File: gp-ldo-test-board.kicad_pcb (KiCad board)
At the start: 2 copper layers, 38.1 x 25.4 mm, 58 parts, among them J1 Conn_01x03, J2 Conn_01x02, J3 Conn_01x06, J4 Conn_01x02, J5 Conn_01x06, J6 Conn_01x02, J7 Conn_01x02, J8 Conn_01x02, J9 Conn_01x02, Q1 Q_PMOS_GSD, U1 SLG46582, U2 SLG46582

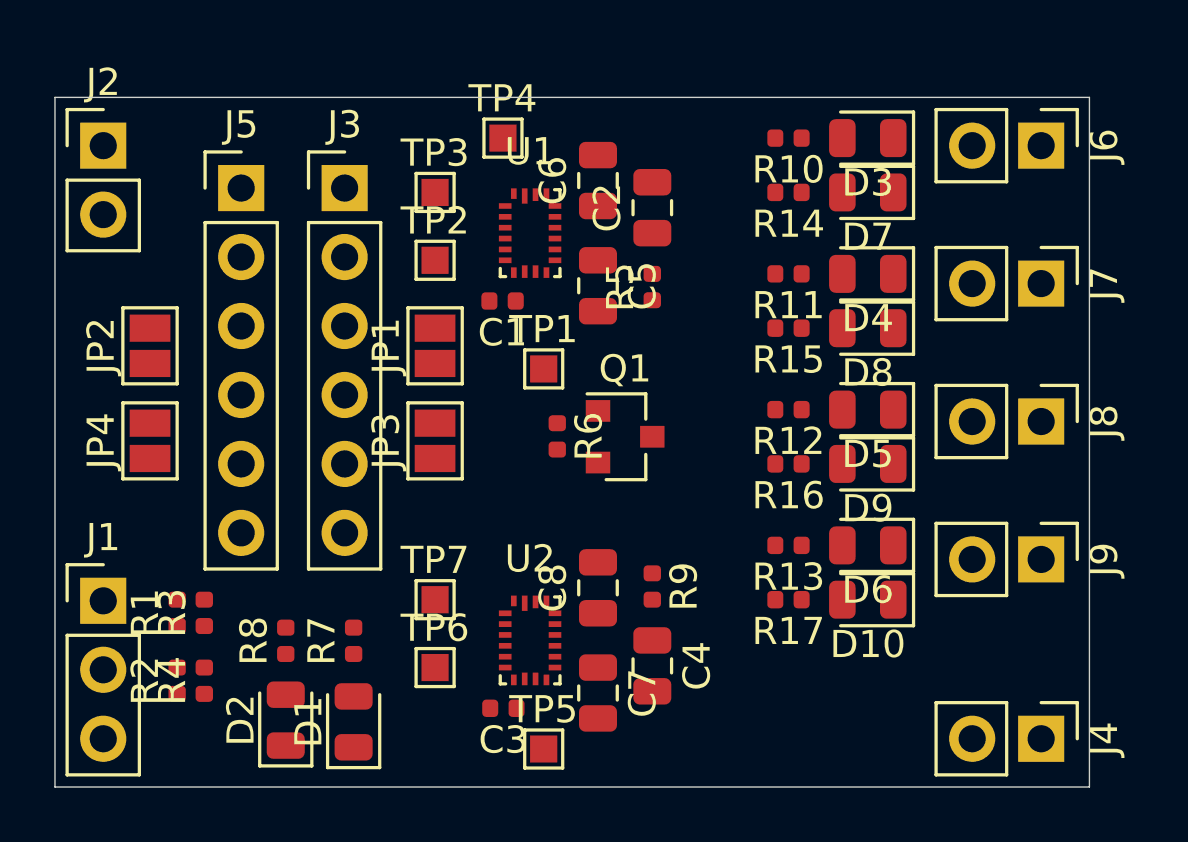
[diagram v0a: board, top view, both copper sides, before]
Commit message: initial route draft
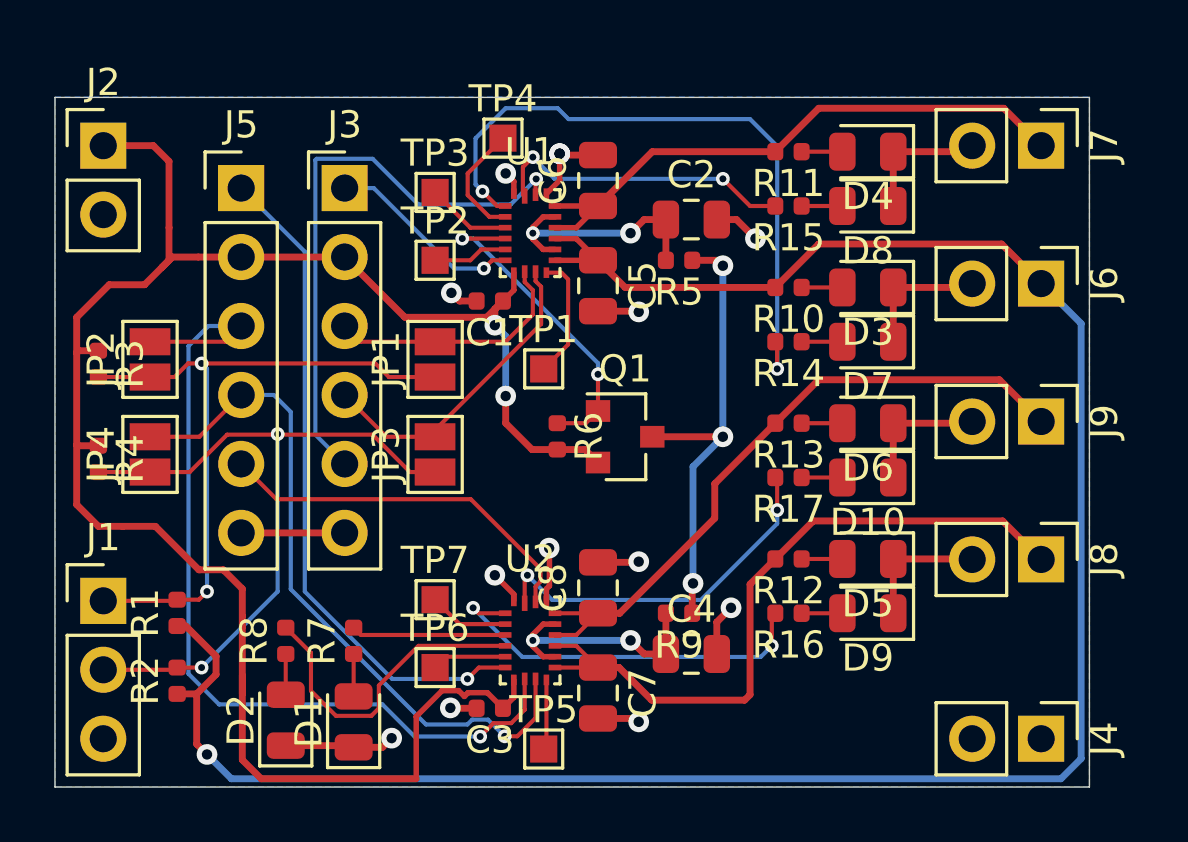
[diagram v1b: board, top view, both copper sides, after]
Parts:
- moved R3 9.96 mm to (51.6, 59.8), turned to 270 degrees
- moved R4 9.05 mm to (51.6, 63.3), turned to 270 degrees
- moved D3 5.50 mm to (79.9, 57.0)
- moved D5 5.50 mm to (79.9, 67.0)
- moved D7 5.50 mm to (79.9, 59.0)
- moved D9 5.50 mm to (79.9, 69.0)
- moved R10 5.50 mm to (77.0, 57.0)
- moved R12 5.50 mm to (77.0, 67.0)
- moved R14 5.50 mm to (77.0, 59.0)
- moved R16 5.50 mm to (77.0, 69.0)
- moved J6 5.08 mm to (86.3, 56.9)
- moved J7 5.08 mm to (86.3, 51.8)
- moved J8 5.08 mm to (86.3, 67.0)
- moved J9 5.08 mm to (86.3, 61.9)
- moved D10 4.50 mm to (79.9, 64.0)
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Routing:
- net /V_3.3_MGMT: track 0.00 -> 79.2 mm, vias 0 -> 1
- net +5V: track 0.00 -> 71.5 mm, vias 0 -> 2
- net GND: track 0.00 -> 45.1 mm, vias 0 -> 13
- net /SLG1_SCL: track 0.00 -> 32.8 mm, vias 0 -> 1
- net /CTRL_SDA: track 0.00 -> 27.0 mm, vias 0 -> 2
- net /V_Vccio1: track 0.00 -> 26.0 mm
- net /SLG1_SDA: track 0.00 -> 25.7 mm, vias 0 -> 1
- net /CTRL_SCL: track 0.00 -> 25.3 mm, vias 0 -> 2
- net /V_Vccio2: track 0.00 -> 24.8 mm
- net Net-(J5-Pad1): track 0.00 -> 24.7 mm, vias 0 -> 1
- net /V_3.3_MGMT_FAULT: track 0.00 -> 24.5 mm, vias 0 -> 2
- net /V_1.8_Vcore: track 0.00 -> 21.9 mm
- net Net-(J3-Pad5): track 0.00 -> 21.5 mm, vias 0 -> 1
- net Net-(Q1-Pad3): track 0.00 -> 17.1 mm, vias 0 -> 3
- net /V_Vccio1_FAULT: track 0.00 -> 14.4 mm, vias 0 -> 2
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- added copper zone on B.Cu, net GND
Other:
- net class power added: clearance 0.1524, trace_width 0.254, via_dia 0.762, via_drill 0.381

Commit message: route major cleanup
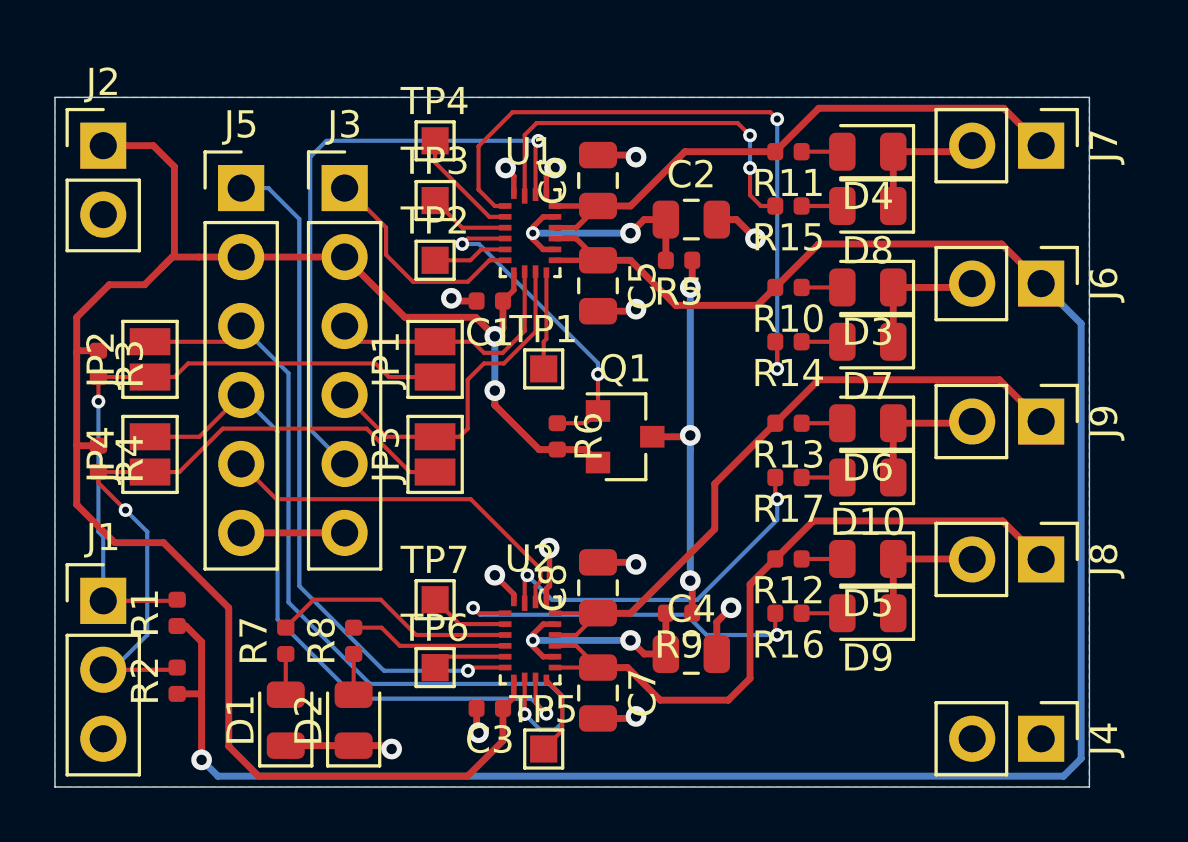
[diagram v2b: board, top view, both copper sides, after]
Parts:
- moved TP4 2.50 mm to (64.0, 51.6)
- moved D1 2.50 mm to (58.5, 72.9)
- moved D2 2.50 mm to (61.0, 72.9)
- moved R7 2.50 mm to (58.5, 70.0)
- moved R8 2.50 mm to (61.0, 70.0)
- moved TP3 0.30 mm to (64.0, 53.8)
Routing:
- net /AUX_LED_1: track 11.8 -> 5.86 mm
- net /AUX_LED_0: track 5.69 -> 9.05 mm
- net +5V: track 71.5 -> 68.5 mm
- net /V_1.8_Vcore_FAULT: track 11.3 -> 14.2 mm
- net /SLG1_SCL: track 32.8 -> 30.0 mm
- net Net-(Q1-Pad3): track 17.1 -> 14.5 mm
- net /CTRL_SDA: track 27.0 -> 25.4 mm, vias 2 -> 1
- net /CTRL_SCL: track 25.3 -> 23.9 mm, vias 2 -> 1
- net Net-(J3-Pad5): track 21.5 -> 22.5 mm
- net Net-(J3-Pad1): track 7.26 -> 8.26 mm, vias 1 -> 0
- net Net-(TP1-Pad1): track 4.57 -> 3.59 mm
- net GND: track 45.1 -> 44.3 mm
- net /SLG0_SDA: track 11.8 -> 12.5 mm
- net /V_Vccio1_FAULT: track 14.4 -> 13.7 mm
